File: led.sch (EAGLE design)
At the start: 22 parts, among them U1 TPS92513HV

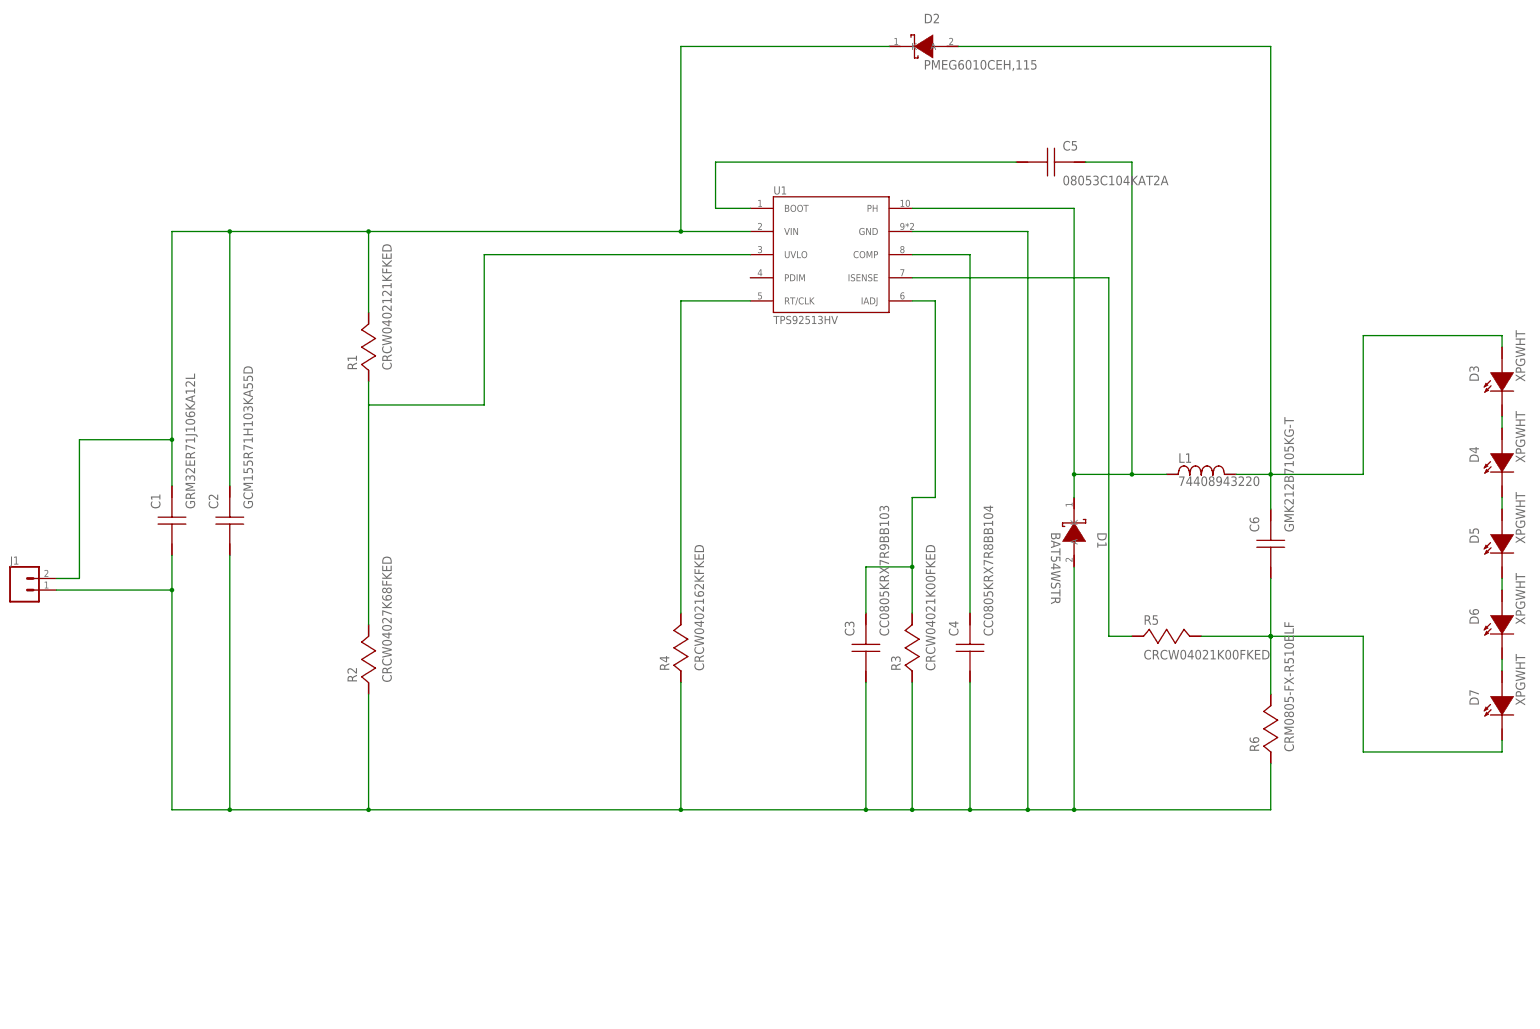
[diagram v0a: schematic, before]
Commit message: save
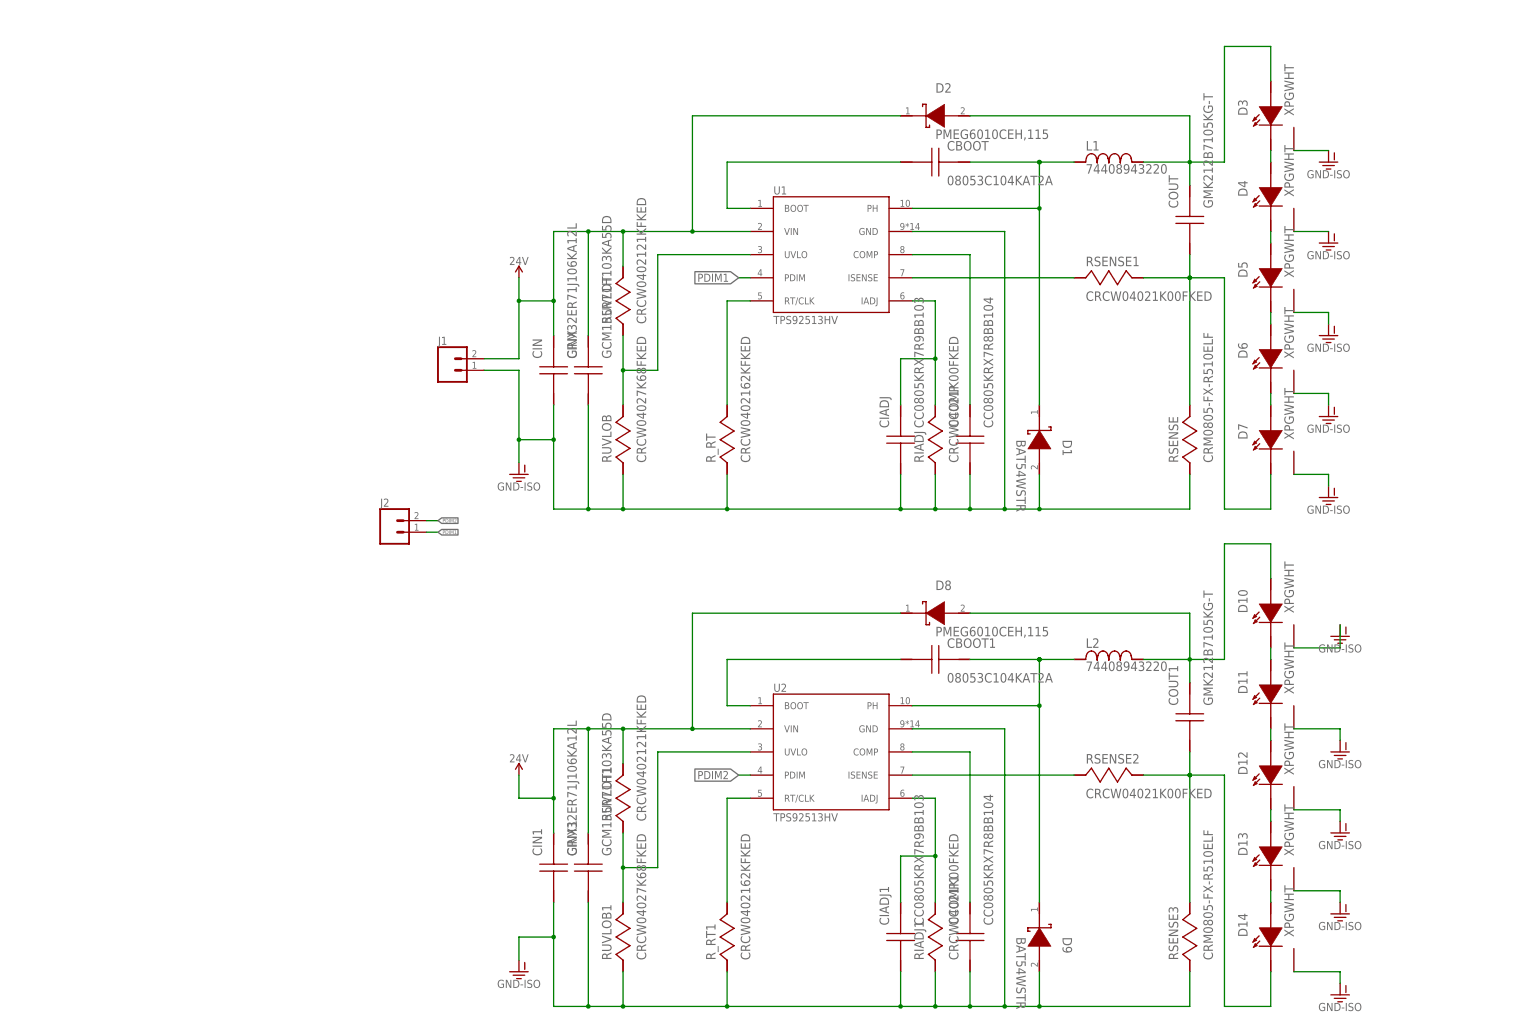
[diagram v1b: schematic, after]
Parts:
- removed C1: GRM32ER71J106KA12L, derek:GRM32ER71J106KA12L
- removed C2: GCM155R71H103KA55D, derek:GCM155R71H103KA55D
- removed C3: CC0805KRX7R9BB103, derek:CC0805KRX7R9BB103
- removed C4: CC0805KRX7R8BB104, derek:CC0805KRX7R8BB104
- removed C5: 08053C104KAT2A, derek:08053C104KAT2A
- removed C6: GMK212B7105KG-T, derek:GMK212B7105KG-T
- removed R1: CRCW0402121KFKED, derek:CRCW0402121KFKED
- removed R2: CRCW04027K68FKED, derek:CRCW04027K68FKED
- removed R3, R5: CRCW04021K00FKED, derek:CRCW04021K00FKED
- removed R4: CRCW0402162KFKED, derek:CRCW0402162KFKED
- removed R6: CRM0805-FX-R510ELF, derek:CRM0805-FX-R510ELF
- added CBOOT, CBOOT1: 08053C104KAT2A, derek:08053C104KAT2A
- added CCOMP, CCOMP1: CC0805KRX7R8BB104, derek:CC0805KRX7R8BB104
- added CIADJ, CIADJ1: CC0805KRX7R9BB103, derek:CC0805KRX7R9BB103
- added CIN, CIN1: GRM32ER71J106KA12L, derek:GRM32ER71J106KA12L
- added CINX, CINX1: GCM155R71H103KA55D, derek:GCM155R71H103KA55D
- added COUT, COUT1: GMK212B7105KG-T, derek:GMK212B7105KG-T
- added D10, D11, D12, D13, D14: XPGWHT, derek:XPGWHT
- added D8: PMEG6010CEH,115, derek:PMEG6010CEH,115
- added D9: BAT54WSTR, derek:BAT54WSTR
- added J2: (no value), derek:CONN_02
- added L2: 74408943220, derek:74408943220
- added RIADJ, RIADJ1, RSENSE1, RSENSE2: CRCW04021K00FKED, derek:CRCW04021K00FKED
- added RSENSE, RSENSE3: CRM0805-FX-R510ELF, derek:CRM0805-FX-R510ELF
- added RUVLOB, RUVLOB1: CRCW04027K68FKED, derek:CRCW04027K68FKED
- added RUVLOT, RUVLOT1: CRCW0402121KFKED, derek:CRCW0402121KFKED
- added R_RT, R_RT1: CRCW0402162KFKED, derek:CRCW0402162KFKED
- added U2: TPS92513HV, derek:TPS92513HV
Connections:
- removed net GND: C1.2, C2.2, C3.2, C4.2, D1.A, J1.1, R2.2, R3.2, R4.2, R6.2, U1.GND
- new net 24V: CIN.1, CIN1.1, CINX.1, CINX1.1, D2.C, D8.C, J1.2, RUVLOT.1, RUVLOT1.1, U1.VIN, U2.VIN
- new net GND-ISO: CCOMP.2, CCOMP1.2, CIADJ.2, CIADJ1.2, CIN.2, CIN1.2, CINX.2, CINX1.2, D1.A, D10.GND, D11.GND, D12.GND, D13.GND, D14.GND, D3.GND, D4.GND, D5.GND, D6.GND, D7.GND, D9.A, J1.1, RIADJ.2, RIADJ1.2, RSENSE.2, RSENSE3.2, RUVLOB.2, RUVLOB1.2, R_RT.2, R_RT1.2, U1.GND, U2.GND
- new net N$1: RUVLOB1.1, RUVLOT1.2, U2.UVLO
- new net N$16: CBOOT1.1, D9.C, L2.1, U2.PH
- new net N$17: COUT1.2, D14.C, RSENSE2.1, RSENSE3.1
- new net N$18: COUT1.1, D10.A, D8.A, L2.2
- new net N$19: R_RT1.1, U2.RT/CLK
- new net N$20: CCOMP1.1, U2.COMP
- new net N$21: CBOOT1.2, U2.BOOT
- new net N$22: RSENSE2.2, U2.ISENSE
- new net N$23: D10.C, D11.A
- new net N$24: D11.C, D12.A
- new net N$25: D12.C, D13.A
- new net N$26: D13.C, D14.A
- new net PDIM1: J2.1, U1.PDIM
- new net PDIM2: J2.2, U2.PDIM
- net N$10: now also CBOOT.2; no longer C5.2
- net N$11: now also RSENSE1.2; no longer R5.2
- net N$2: now also CIADJ.1, RIADJ.1; no longer C3.1, R3.1
- net N$3: now also RUVLOB.1, RUVLOT.2; no longer R1.2, R2.1
- net N$4: now also CIADJ1.1, RIADJ1.1, U2.IADJ; no longer C1.1, C2.1, D2.K, J1.2, R1.1, U1.VIN
- net N$5: now also CBOOT.1, D1.C; no longer C5.1, D1.K
- net N$6: now also COUT.2, RSENSE.1, RSENSE1.1; no longer C6.2, R5.1, R6.1
- net N$7: now also COUT.1; no longer C6.1
- net N$8: now also R_RT.1; no longer R4.1
- net N$9: now also CCOMP.1; no longer C4.1
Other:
- moved on the sheet: J1, L1, U1
